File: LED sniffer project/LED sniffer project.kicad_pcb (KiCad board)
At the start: 2 copper layers, 220.5 x 147 mm, 13 parts, among them J1 Conn_01x02_Pin, Q1 2N3904, SW1 Push_Button

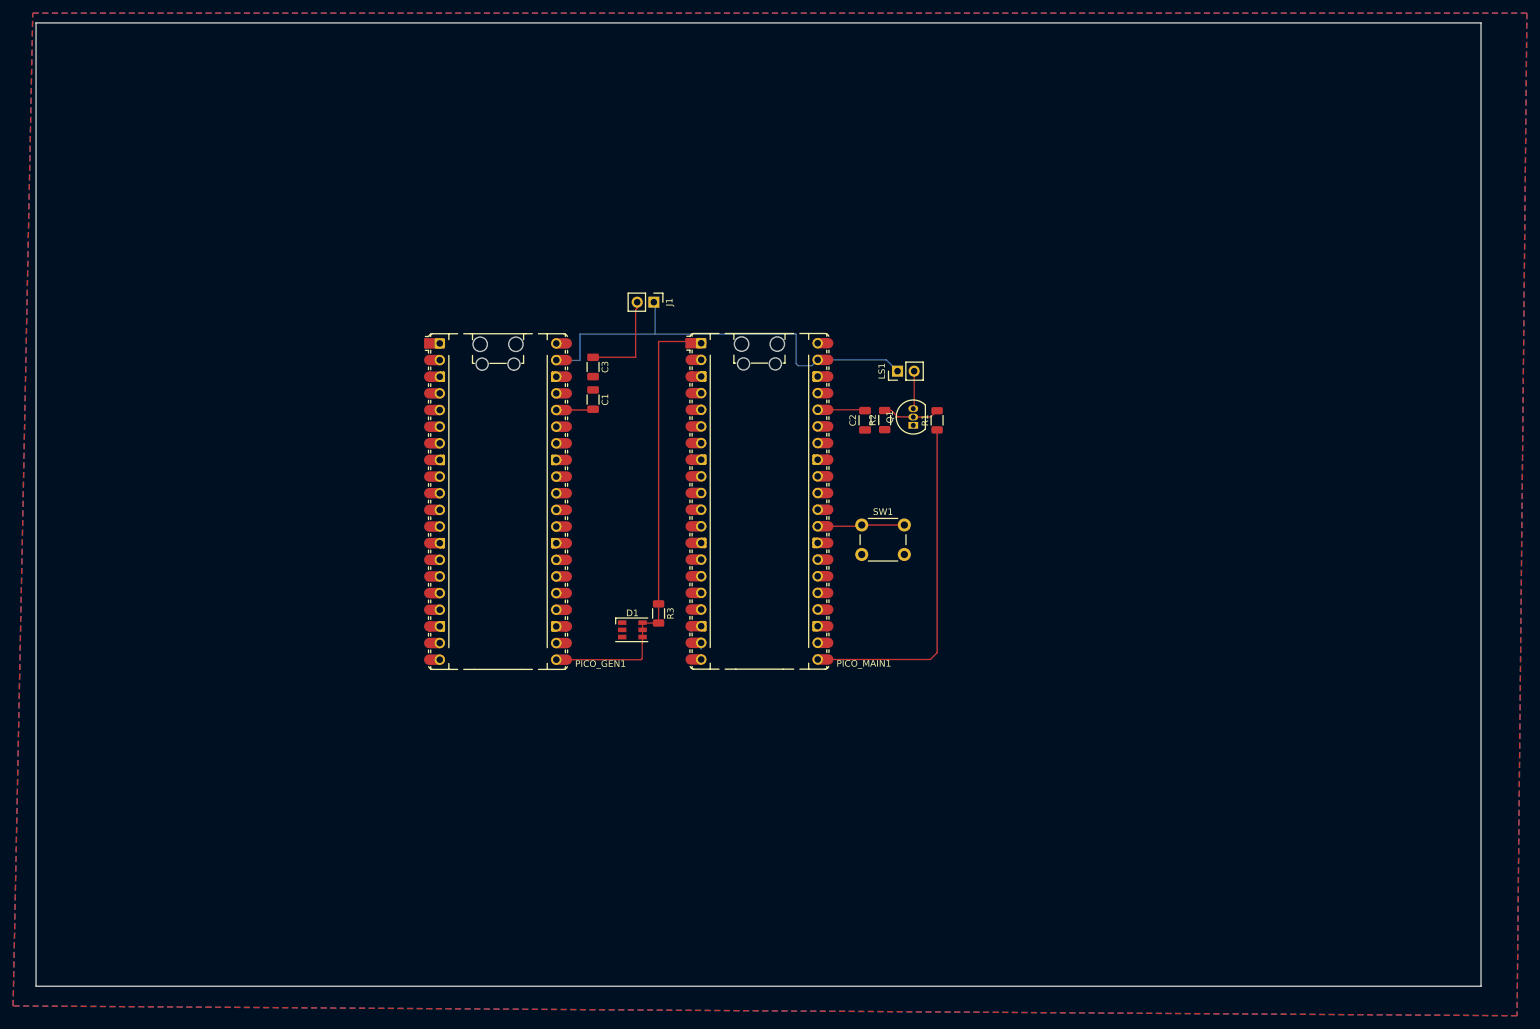
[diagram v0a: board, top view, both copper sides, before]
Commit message: rough draft of schematic
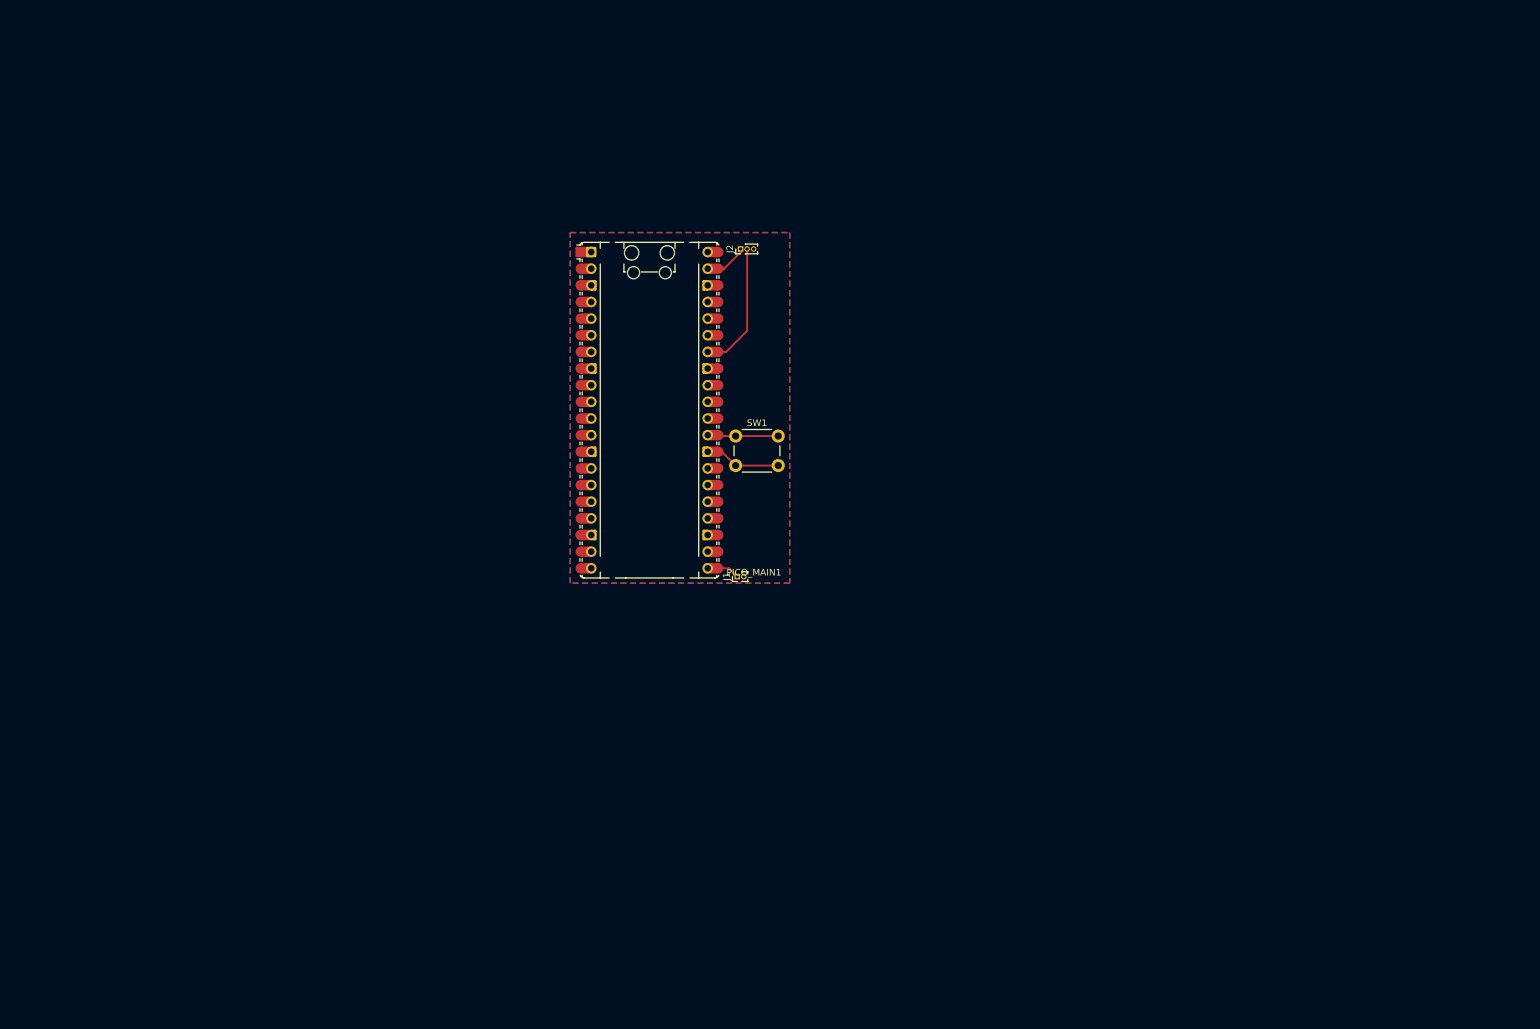
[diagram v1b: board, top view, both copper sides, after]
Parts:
- removed C1, C2: 0.1u, Capacitor_SMD:C_1206_3216Metric
- removed C3: 50u, Capacitor_SMD:C_1206_3216Metric
- removed D1: LED_RGB, LED_SMD:LED_RGB_PLCC-6
- removed LS1: Speaker, Connector_PinHeader_2.54mm:PinHeader_1x02_P2.54mm_Vertical
- removed PICO_GEN1: RaspberryPi_Pico, Module:RaspberryPi_Pico_Common_Unspecified
- removed Q1: 2N3904, Package_TO_SOT_THT:TO-92_Inline
- removed R1: 1k, Resistor_SMD:R_1206_3216Metric
- removed R2: 100k, Resistor_SMD:R_1206_3216Metric
- removed R3: 330, Resistor_SMD:R_1206_3216Metric
- added J2: Conn_01x03, Connector_PinHeader_1.00mm:PinHeader_1x03_P1.00mm_Vertical, F.Cu at (151.0, 52.5)
- J1: value Conn_01x02_Pin -> Conn_01x02; footprint Connector_PinHeader_2.54mm:PinHeader_1x02_P2.54mm_Vertical -> Connector_PinHeader_1.00mm:PinHeader_1x02_P1.00mm_Vertical
- moved J1 43.8 mm to (150.5, 102.5), turned to 90 degrees
- moved SW1 23.5 mm to (150.3, 81.0)
- moved PICO_MAIN1 21.8 mm to (137.1, 77.1)
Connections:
- J1 pad 1: 5V -> Net-(J1-Pin_1)
- J1 pad 2: Net-(J1-Pin_2) -> GND
- PICO_MAIN1 pad 1: /Din -> unconnected-(PICO_MAIN1-GPIO0-Pad1)
- PICO_MAIN1 pad 21: /SPEAKER_OUT -> Net-(J1-Pin_1)
- PICO_MAIN1 pad 36: Net-(PICO_MAIN1-3V3) -> unconnected-(PICO_MAIN1-3V3-Pad36)
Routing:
- net /Din: track 70.7 -> 0.00 mm
- net 5V: track 66.3 -> 7.75 mm
- net /SPEAKER_OUT: track 52.7 -> 0.00 mm
- net unconnected-(J2-Pin_2-Pad2): track 0.00 -> 19.0 mm
- net Net-(J1-Pin_2): track 15.0 -> 0.00 mm
- net GND: track 0.00 -> 10.8 mm
- net Net-(Q1-B): track 8.81 -> 0.00 mm
- net Net-(PICO_MAIN1-3V3): track 7.27 -> 0.00 mm
- net Net-(Q1-C): track 5.79 -> 0.00 mm
- net Net-(PICO_GEN1-3V3): track 5.66 -> 0.00 mm
- net Net-(J1-Pin_1): track 0.00 -> 4.24 mm
- net /BTN_IN: track 13.3 -> 10.0 mm
- net unconnected-(PICO_MAIN1-GPIO14-Pad19): track 0.92 -> 0.00 mm
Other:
- board outline removed

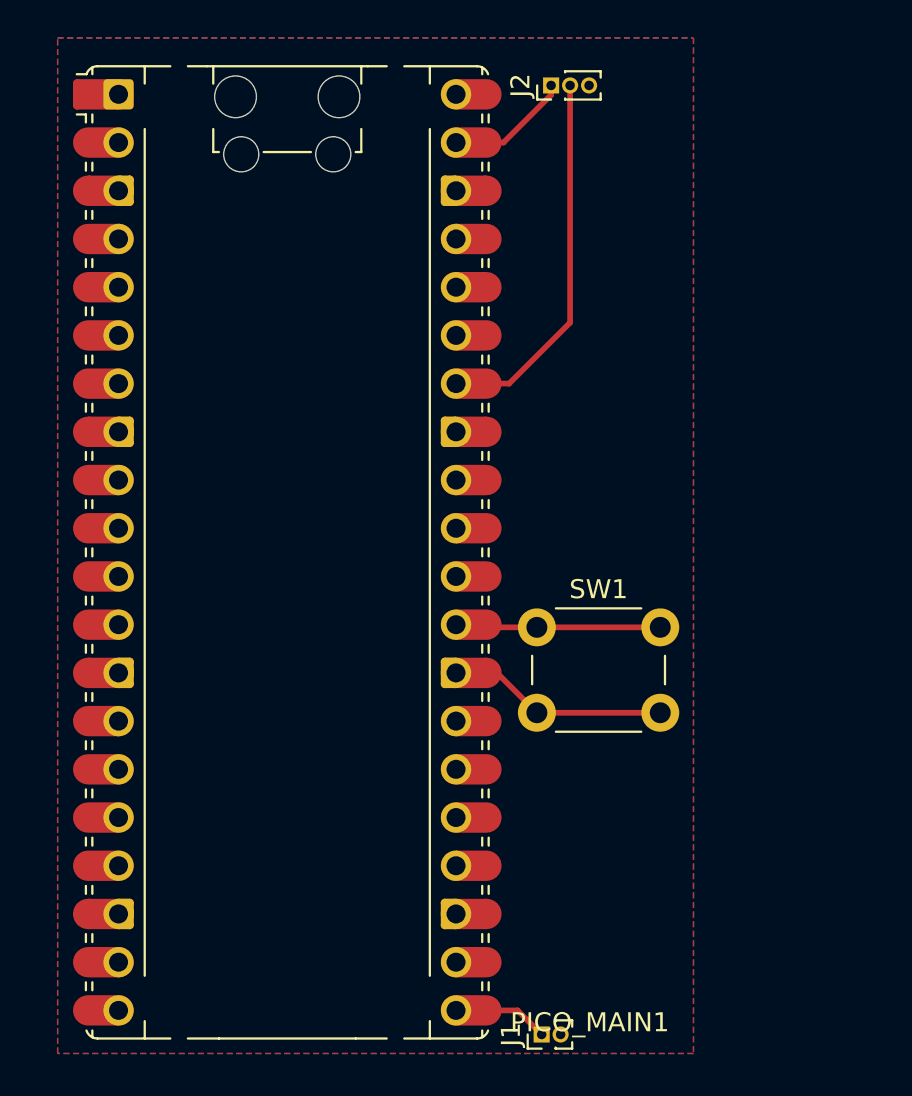
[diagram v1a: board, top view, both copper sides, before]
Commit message: Updated CAD
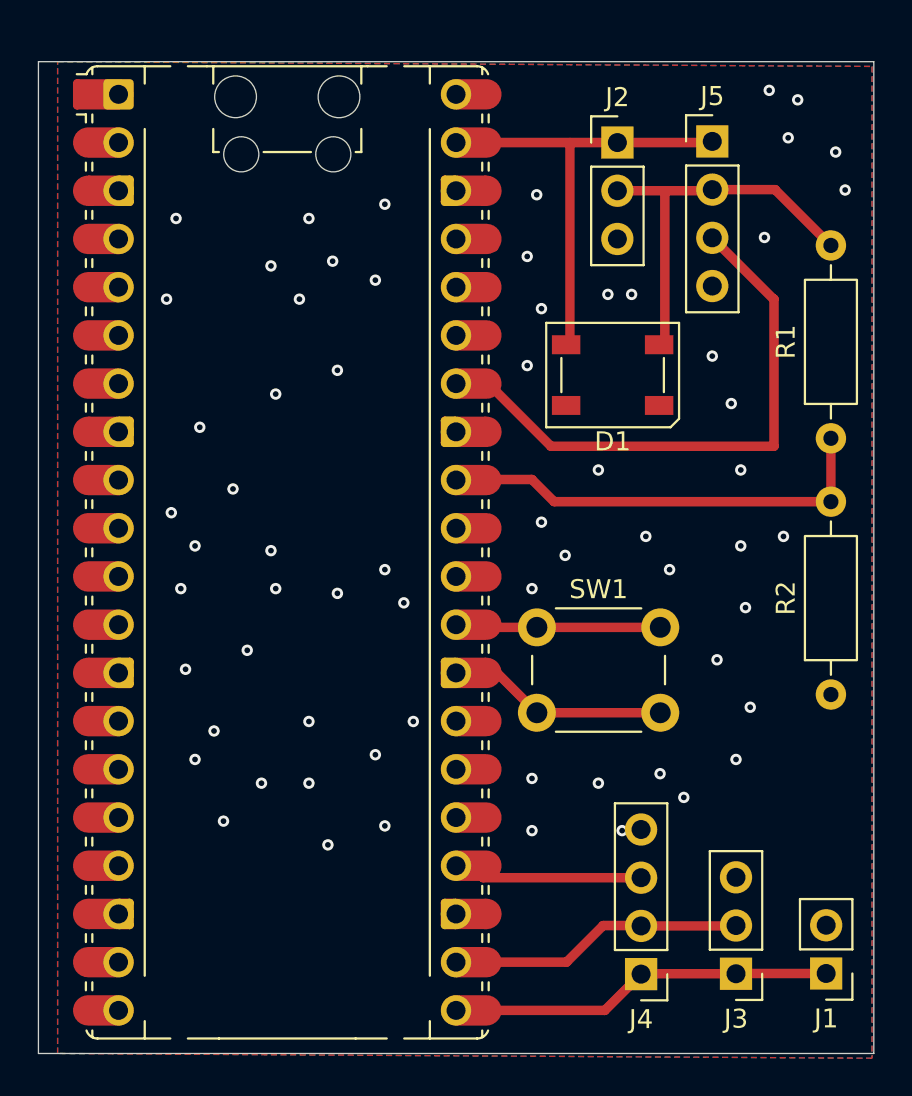
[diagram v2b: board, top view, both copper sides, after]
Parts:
- added D1: SK6812, LED_SMD:LED_SK6812_PLCC4_5.0x5.0mm_P3.2mm, F.Cu at (154.2, 67.8)
- added J3: Conn_01x03, Connector_PinHeader_2.54mm:PinHeader_1x03_P2.54mm_Vertical, F.Cu at (160.8, 99.3)
- added J4: Conn_01x04, Connector_PinHeader_2.54mm:PinHeader_1x04_P2.54mm_Vertical, F.Cu at (155.8, 99.3)
- added J5: Conn_01x04, Connector_PinHeader_2.54mm:PinHeader_1x04_P2.54mm_Vertical, F.Cu at (159.5, 55.4)
- added R1: 22k, Resistor_THT:R_Axial_DIN0207_L6.3mm_D2.5mm_P10.16mm_Horizontal, F.Cu at (165.8, 71.1)
- added R2: 33k, Resistor_THT:R_Axial_DIN0207_L6.3mm_D2.5mm_P10.16mm_Horizontal, F.Cu at (165.8, 84.6)
- J1: footprint Connector_PinHeader_1.00mm:PinHeader_1x02_P1.00mm_Vertical -> Connector_PinHeader_2.54mm:PinHeader_1x02_P2.54mm_Vertical
- J2: footprint Connector_PinHeader_1.00mm:PinHeader_1x03_P1.00mm_Vertical -> Connector_PinHeader_2.54mm:PinHeader_1x03_P2.54mm_Vertical
- moved J1 15.3 mm to (165.5, 99.3), turned to 180 degrees
- moved J2 4.61 mm to (154.5, 55.5), turned to 0 degrees
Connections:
- J2 pad 2: unconnected-(J2-Pin_2-Pad2) -> Net-(D1-DIN)
- PICO_MAIN1 pad 22: unconnected-(PICO_MAIN1-GPIO17-Pad22) -> Net-(J3-Pin_2)
- PICO_MAIN1 pad 24: unconnected-(PICO_MAIN1-GPIO18-Pad24) -> Net-(J4-Pin_3)
- PICO_MAIN1 pad 32: unconnected-(PICO_MAIN1-GPIO27_ADC1-Pad32) -> Net-(PICO_MAIN1-GPIO27_ADC1)
- PICO_MAIN1 pad 34: unconnected-(J2-Pin_2-Pad2) -> Net-(J5-Pin_3)
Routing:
- net Net-(J5-Pin_3): track 0.00 -> 30.5 mm
- net Net-(PICO_MAIN1-GPIO27_ADC1): track 0.00 -> 23.6 mm
- net Net-(D1-DIN): track 0.00 -> 20.7 mm
- net unconnected-(J2-Pin_2-Pad2): track 19.0 -> 0.00 mm
- net 5V: track 7.75 -> 23.5 mm
- net Net-(J1-Pin_1): track 4.24 -> 19.9 mm
- net Net-(J3-Pin_2): track 0.00 -> 14.8 mm
- net Net-(J4-Pin_3): track 0.00 -> 9.21 mm
- net unconnected-(PICO_MAIN1-3V3_EN-Pad37)_1: track 0.00 -> 1.71 mm
- net GND: vias 0 -> 65
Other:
- board outline added: 44 x 52.2 mm
- board text added: "Team 09"
